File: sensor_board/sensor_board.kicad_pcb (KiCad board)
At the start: 2 copper layers, 88.9 x 95.2 mm, 36 parts, among them J1 Conn_02x20_Odd_Even, J2 Conn_Coaxial, J3 Conn_Coaxial, U1 BME280, U2 MPU-6050, U3 NEO-7M-0, U4 RFM95W-868S2

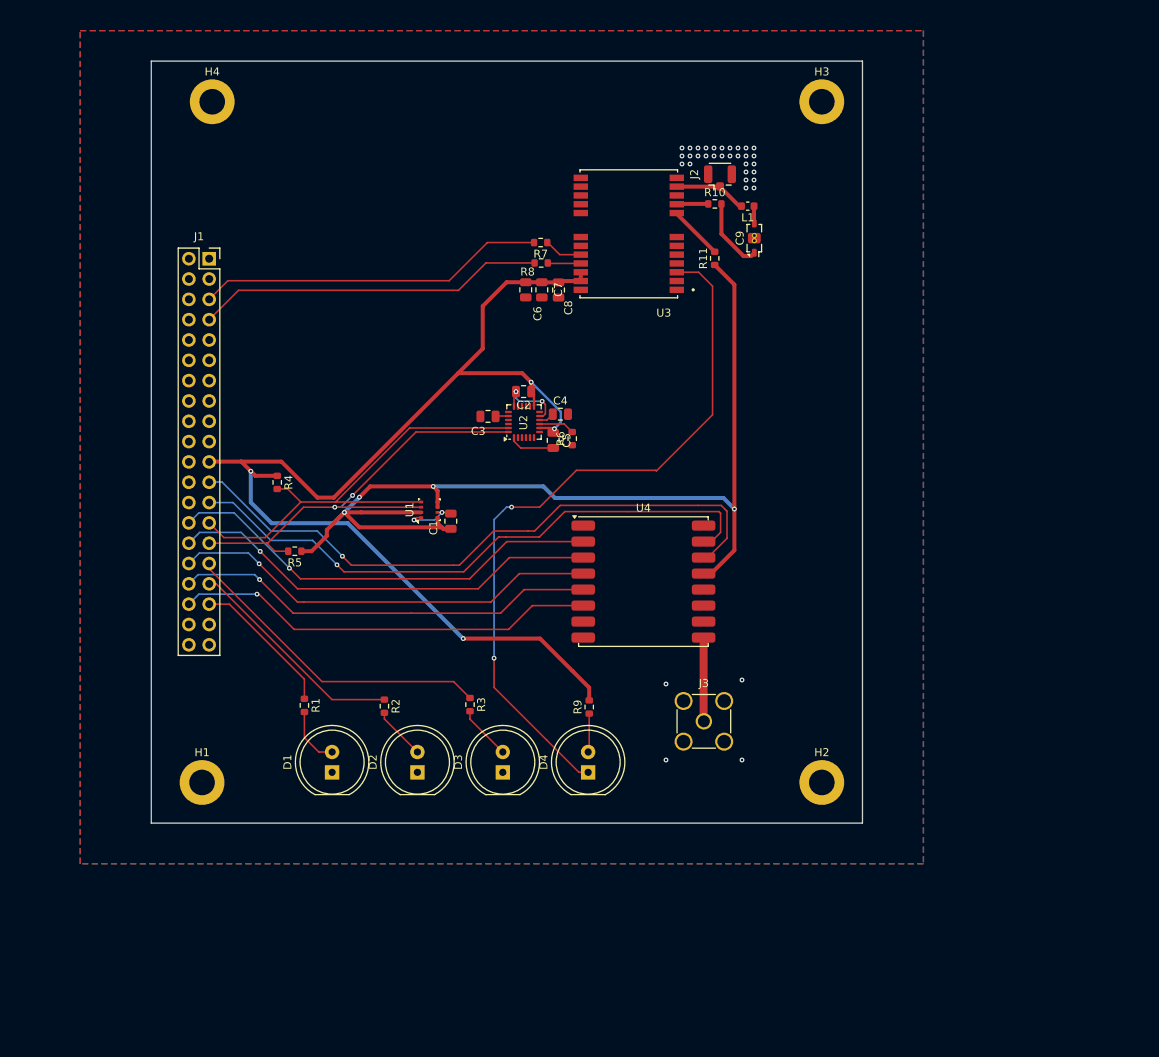
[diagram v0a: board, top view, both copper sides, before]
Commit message: sensor
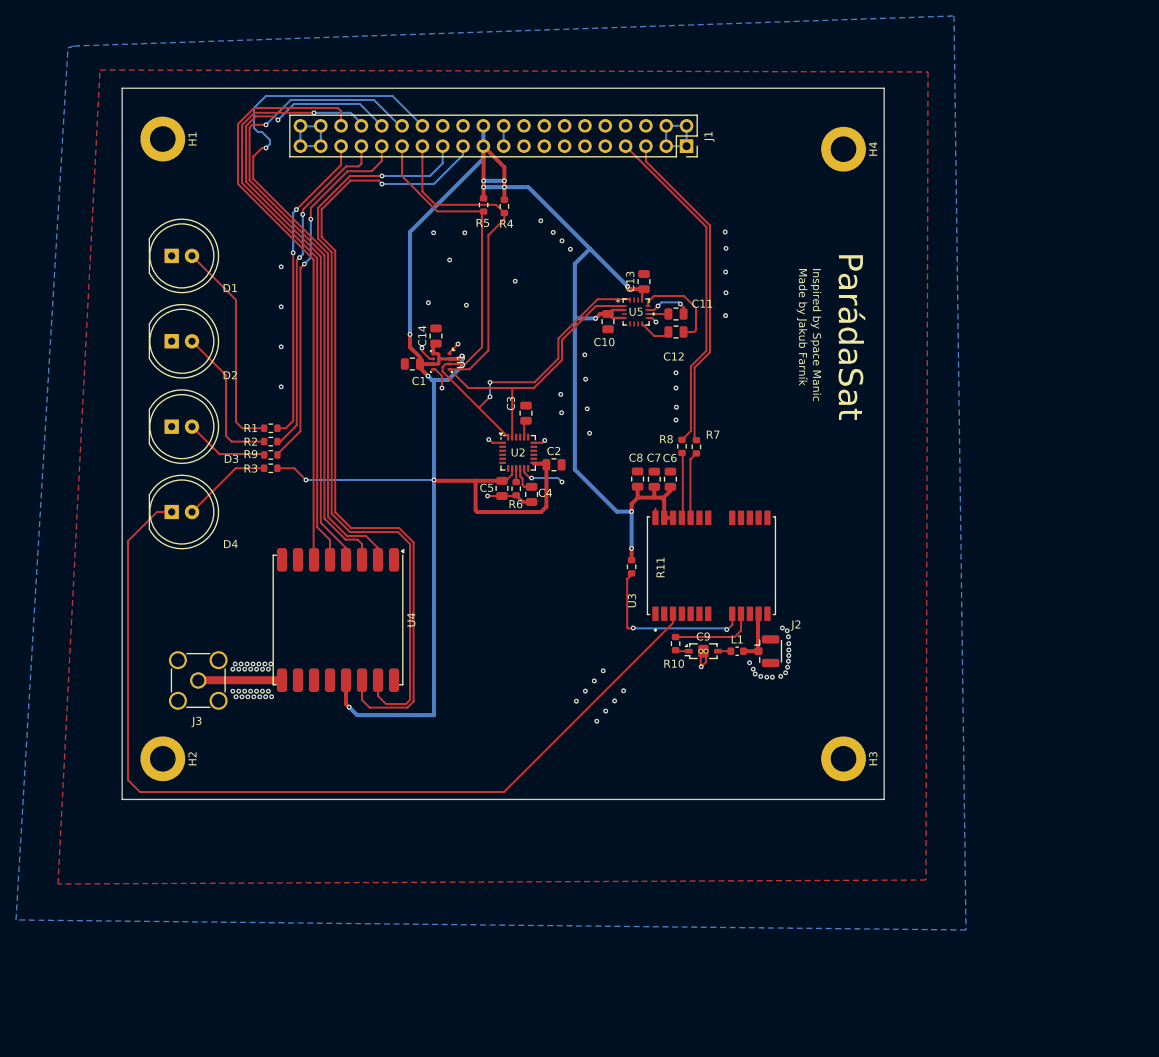
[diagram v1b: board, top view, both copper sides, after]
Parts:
- added C10: 0.1uF, Capacitor_SMD:C_0805_2012Metric, F.Cu at (130.8, 73.2)
- added C11: 4.7uF, Capacitor_SMD:C_0805_2012Metric, F.Cu at (139.2, 72.2)
- added C12: 0.22uF, Capacitor_SMD:C_0805_2012Metric, F.Cu at (139.2, 74.5)
- added C13: 0.1uF, Capacitor_SMD:C_0805_2012Metric, F.Cu at (135.2, 68.2)
- added C14: 0.1uF, Capacitor_SMD:C_0805_2012Metric, F.Cu at (109.2, 75.0)
- added U5: HMC5883L, footprints:LPCC16_HNW, F.Cu at (134.3, 72.0)
- moved H2 82.4 mm to (75.1, 127.8), turned to -90 degrees
- moved H3 82.2 mm to (160.2, 127.8), turned to -90 degrees
- moved H1 80.6 mm to (75.1, 50.4), turned to -90 degrees
- moved H4 79.1 mm to (160.2, 51.6), turned to -90 degrees
- moved D1 67.6 mm to (76.2, 65.0), turned to 0 degrees
- moved J3 63.4 mm to (79.5, 118.1), turned to -90 degrees
- moved D2 62.0 mm to (76.2, 75.7), turned to 0 degrees
- moved D4 61.4 mm to (76.2, 97.0), turned to 0 degrees
- moved J1 61.3 mm to (140.6, 51.3), turned to -90 degrees
- moved D3 59.8 mm to (76.2, 86.3), turned to 0 degrees
- moved J2 59.4 mm to (150.6, 114.4), turned to 0 degrees
- moved L1 55.6 mm to (146.9, 114.4), turned to 0 degrees
- moved R10 55.2 mm to (139.2, 113.5), turned to -90 degrees
- moved C9 52.0 mm to (142.7, 114.4), turned to 0 degrees
- moved R9 49.7 mm to (88.6, 91.5), turned to 0 degrees
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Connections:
- U1 pad 5: +3V3 -> GND
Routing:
- net MISO: track 55.2 -> 89.8 mm
- net GND: track 21.1 -> 54.6 mm, vias 38 -> 93
- net MOSI: track 54.4 -> 82.5 mm
- net SCK: track 53.8 -> 79.0 mm
- net PPS: track 91.2 -> 115.5 mm, vias 2 -> 0
- net NSS: track 53.0 -> 75.3 mm
- net DIO0: track 79.8 -> 101.4 mm
- net RST: track 52.9 -> 74.2 mm, vias 1 -> 0
- net LED_SUCCESS: track 18.2 -> 39.2 mm, vias 0 -> 2
- net DIO1: track 75.7 -> 96.4 mm
- net SDA: track 57.1 -> 77.8 mm
- net Net-(D1-A): track 7.41 -> 26.9 mm
- net SCL: track 58.2 -> 75.5 mm
- net Net-(U3-RESET_N): track 6.80 -> 22.0 mm, vias 0 -> 2
- net LED_WARN: track 27.9 -> 42.4 mm, vias 0 -> 2
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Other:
- board size 88.9 x 95.2 mm -> 95.3 x 88.9 mm
- board text added: "Inspired by Space Manic"
- board text added: "Made by Jakub Farník"
- board text added: "ParádaSat"

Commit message: completed sensor
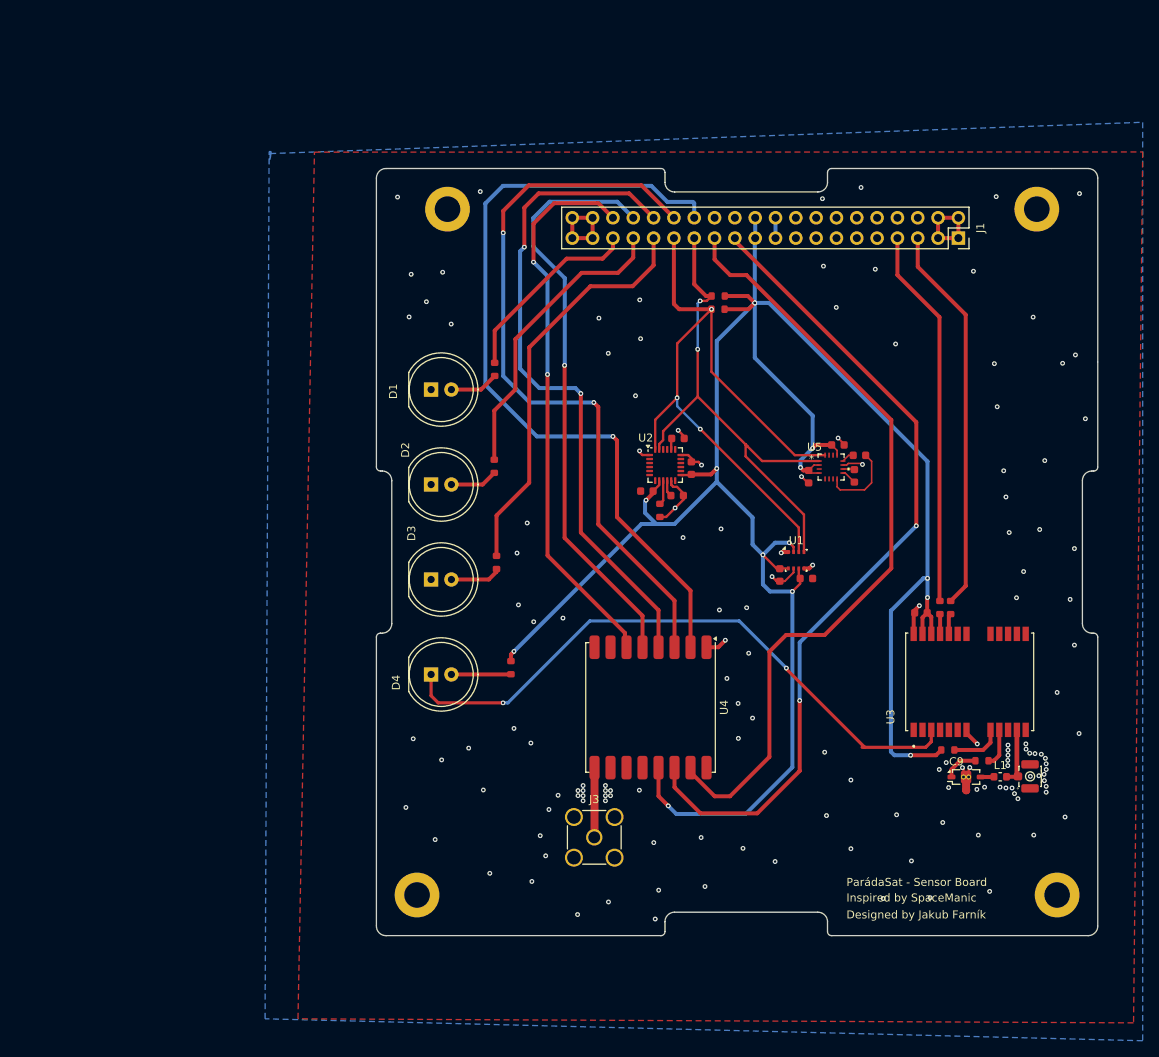
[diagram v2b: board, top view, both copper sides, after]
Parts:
- removed C1, C13, C14, C5: 0.1uF, Capacitor_SMD:C_0805_2012Metric
- removed C12: 0.22uF, Capacitor_SMD:C_0805_2012Metric
- removed C3: 2.2nF, Capacitor_SMD:C_0805_2012Metric
- removed C6: 10uF, Capacitor_SMD:C_0805_2012Metric
- removed C7: 1uF, Capacitor_SMD:C_0805_2012Metric
- removed C8: 100nF, Capacitor_SMD:C_0805_2012Metric
- removed H1, H2, H3, H4: MountingHole_Pad, MountingHole:MountingHole_3.2mm_M3_DIN965_Pad
- removed J2: Conn_Coaxial, Connector_Coaxial:U.FL_Hirose_U.FL-R-SMT-1_Vertical
- removed R11: 10k, Resistor_SMD:R_0603_1608Metric
- added C15: 100nF, PCM_JLCPCB:C_0603, F.Cu at (155.8, 92.6)
- added C16: 100nF, PCM_JLCPCB:C_0603, F.Cu at (159.5, 88.6)
- added C17: 100nF, PCM_JLCPCB:C_0603, F.Cu at (139.4, 94.9)
- added C18: 100nF, PCM_JLCPCB:C_0603, F.Cu at (135.6, 94.4)
- added C19: 100nF, PCM_JLCPCB:C_0603, F.Cu at (141.2, 91.5)
- added C20: 100nF, PCM_JLCPCB:C_0603, F.Cu at (152.2, 104.9)
- added C21: 100nF, PCM_JLCPCB:C_0603, F.Cu at (155.5, 105.3)
- added J4: U.FL, PCM_JLCPCB:IPEX-SMD_BWIPX-1-001E, F.Cu at (182.8, 130.0)
- added M1: HOLE, MountingHole:MountingHole_3.2mm_M3_DIN965_Pad, F.Cu at (110.7, 59.1)
- added M2: HOLE, MountingHole:MountingHole_3.2mm_M3_DIN965_Pad, F.Cu at (186.9, 144.9)
- added M3: HOLE, MountingHole:MountingHole_3.2mm_M3_DIN965_Pad, F.Cu at (106.9, 144.9)
- added M4: HOLE, MountingHole:MountingHole_3.2mm_M3_DIN965_Pad, F.Cu at (184.4, 59.1)
- added R14: 330Ω, PCM_JLCPCB:R_0603, F.Cu at (116.8, 103.3)
- C10: value 0.1uF -> 470nF; footprint Capacitor_SMD:C_0805_2012Metric -> PCM_JLCPCB:C_0603
- C11: value 4.7uF -> 220nF; footprint Capacitor_SMD:C_0805_2012Metric -> PCM_JLCPCB:C_0603
- C2: value 0.1uF -> 10uF; footprint Capacitor_SMD:C_0805_2012Metric -> PCM_JLCPCB:C_0603
- C4: value 0.1uF -> 2.2nF; footprint Capacitor_SMD:C_0805_2012Metric -> PCM_JLCPCB:C_0603
- R1: value 220 -> 4.7kΩ; footprint Resistor_SMD:R_0603_1608Metric -> PCM_JLCPCB:R_0603
- R10: value 10R -> 10kΩ; footprint Resistor_SMD:R_0603_1608Metric -> PCM_JLCPCB:R_0603
- R2: value 220 -> 10Ω; footprint Resistor_SMD:R_0603_1608Metric -> PCM_JLCPCB:R_0603
- R3: value 220 -> 510Ω; footprint Resistor_SMD:R_0603_1608Metric -> PCM_JLCPCB:R_0603
- R4, R5: value 10K -> 330Ω; footprint Resistor_SMD:R_0603_1608Metric -> PCM_JLCPCB:R_0603
- R6: value 4.7K -> 510Ω; footprint Resistor_SMD:R_0603_1608Metric -> PCM_JLCPCB:R_0603
- R7, R8: value 510R -> 10kΩ; footprint Resistor_SMD:R_0603_1608Metric -> PCM_JLCPCB:R_0603
- R9: value 220R -> 330Ω; footprint Resistor_SMD:R_0603_1608Metric -> PCM_JLCPCB:R_0603
- moved R2 97.4 mm to (177.5, 128.1)
- moved R3 85.8 mm to (172.2, 108.9), turned to 90 degrees
- moved R6 56.3 mm to (173.6, 108.9)
- moved J3 53.2 mm to (129.0, 137.7), turned to 0 degrees
- moved U1 50.8 mm to (154.3, 103.0), turned to 0 degrees
- moved R1 49.7 mm to (137.2, 96.8), turned to -90 degrees
- moved C2 49.5 mm to (169.9, 109.6), turned to 180 degrees
- moved R7 49.2 mm to (173.2, 126.7), turned to 0 degrees
- moved R10 43.8 mm to (144.5, 70.0), turned to 180 degrees
- moved U4 40.6 mm to (136.1, 121.4)
- moved R9 39.0 mm to (118.6, 116.5), turned to -90 degrees
- moved D4 38.3 mm to (108.6, 117.3)
- moved D3 37.6 mm to (108.6, 105.4)
- moved D2 37.0 mm to (108.6, 93.6)
- moved D1 36.5 mm to (108.6, 81.7)
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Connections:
- C10 pad 1: GND -> Net-(U5-C1)
- C10 pad 2: +3V3 -> GND
- C11 pad 1: GND -> Net-(U5-SETC)
- C11 pad 2: Net-(U5-C1) -> Net-(U5-SETP)
- C4 pad 1: Net-(U2-REGOUT) -> Net-(U2-CPOUT)
- R1 pad 1: LED_SUCCESS -> Net-(U2-AD0)
- R1 pad 2: Net-(D1-A) -> GND
- R10 pad 1: VCC_RF -> +3V3
- R10 pad 2: Net-(C9-Pad1) -> SCL
- R2 pad 1: LED_WARN -> VCC_RF
- R2 pad 2: Net-(D2-A) -> Net-(C9-Pad1)
- R3 pad 1: LED_ERROR -> Net-(U3-RXD/SPIMOSI)
- R3 pad 2: Net-(D3-A) -> GPS_RX
- R4 pad 1: +3V3 -> LED_SUCCESS
- R4 pad 2: SCL -> Net-(D1-A)
- R5 pad 1: +3V3 -> LED_WARN
- R5 pad 2: SDA -> Net-(D2-A)
- R6 pad 1: GND -> Net-(U3-TXD/SPIMISO)
- R6 pad 2: Net-(U2-AD0) -> GPS_TX
- R7 pad 1: Net-(U3-TXD/SPIMISO) -> +3V3
- R7 pad 2: GPS_TX -> Net-(U3-RESET_N)
- R8 pad 1: Net-(U3-RXD/SPIMOSI) -> +3V3
- R8 pad 2: GPS_RX -> SDA
- R9 pad 1: Net-(D4-A) -> +3V3
- R9 pad 2: +3V3 -> Net-(D4-A)
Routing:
- net PPS: track 115.5 -> 78.5 mm, vias 0 -> 2
- net Net-(D1-A): track 26.9 -> 6.12 mm
- net Net-(U3-RESET_N): track 22.0 -> 6.49 mm, vias 2 -> 0
- net +3V3: track 269.9 -> 285.3 mm
- net LED_SUCCESS: track 39.2 -> 24.3 mm, vias 2 -> 0
- net Net-(D2-A): track 18.7 -> 5.96 mm
- net MISO: track 89.8 -> 101.4 mm
- net Net-(U5-SETC): track 11.8 -> 1.58 mm
- net MOSI: track 82.5 -> 92.5 mm, vias 1 -> 2
- net SCL: track 75.5 -> 66.4 mm, vias 0 -> 2
- net SDA: track 77.8 -> 85.6 mm, vias 2 -> 3
- net GPS_TX: track 41.0 -> 48.6 mm
- net Net-(U3-TXD/SPIMISO): track 8.37 -> 2.57 mm
- net VCC_RF: track 10.6 -> 4.82 mm
- net Net-(U3-RXD/SPIMOSI): track 8.19 -> 2.48 mm
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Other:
- board size 95.3 x 88.9 mm -> 90.2 x 95.9 mm
- board text added: "Designed by Jakub Farník"
- board text added: "Inspired by SpaceManic"
- board text added: "JLCJLCJLCJLC"
- board text added: "ParádaSat - Sensor Board"
- board text removed: "Inspired by Space Manic"
- board text removed: "Made by Jakub Farník"
- board text removed: "ParádaSat"
